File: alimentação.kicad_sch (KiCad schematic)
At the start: 10 parts, among them U2 LM317G, U3 AMS1117-5.0

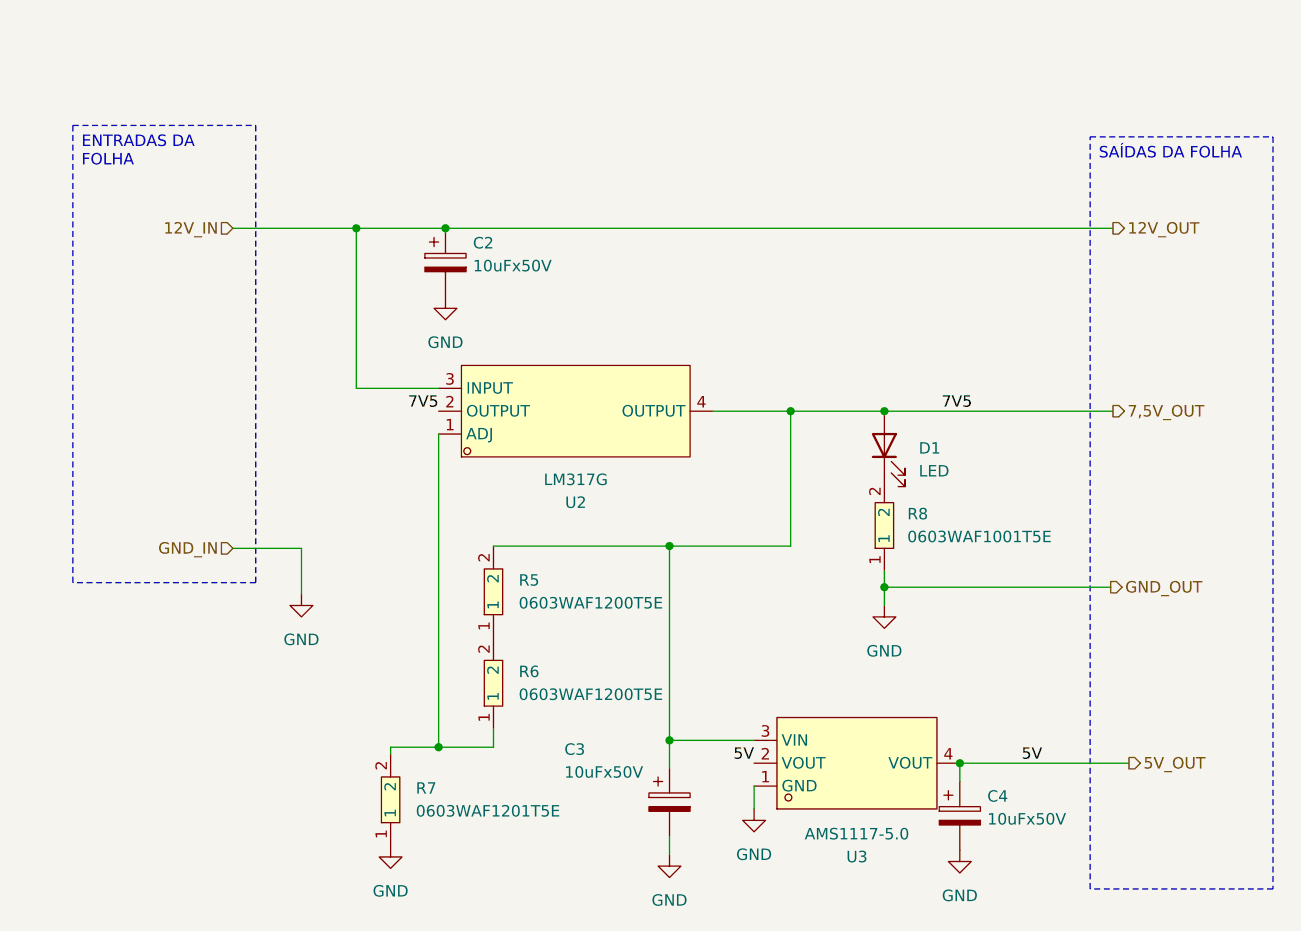
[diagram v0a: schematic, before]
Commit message: organização e legendas do esquemático
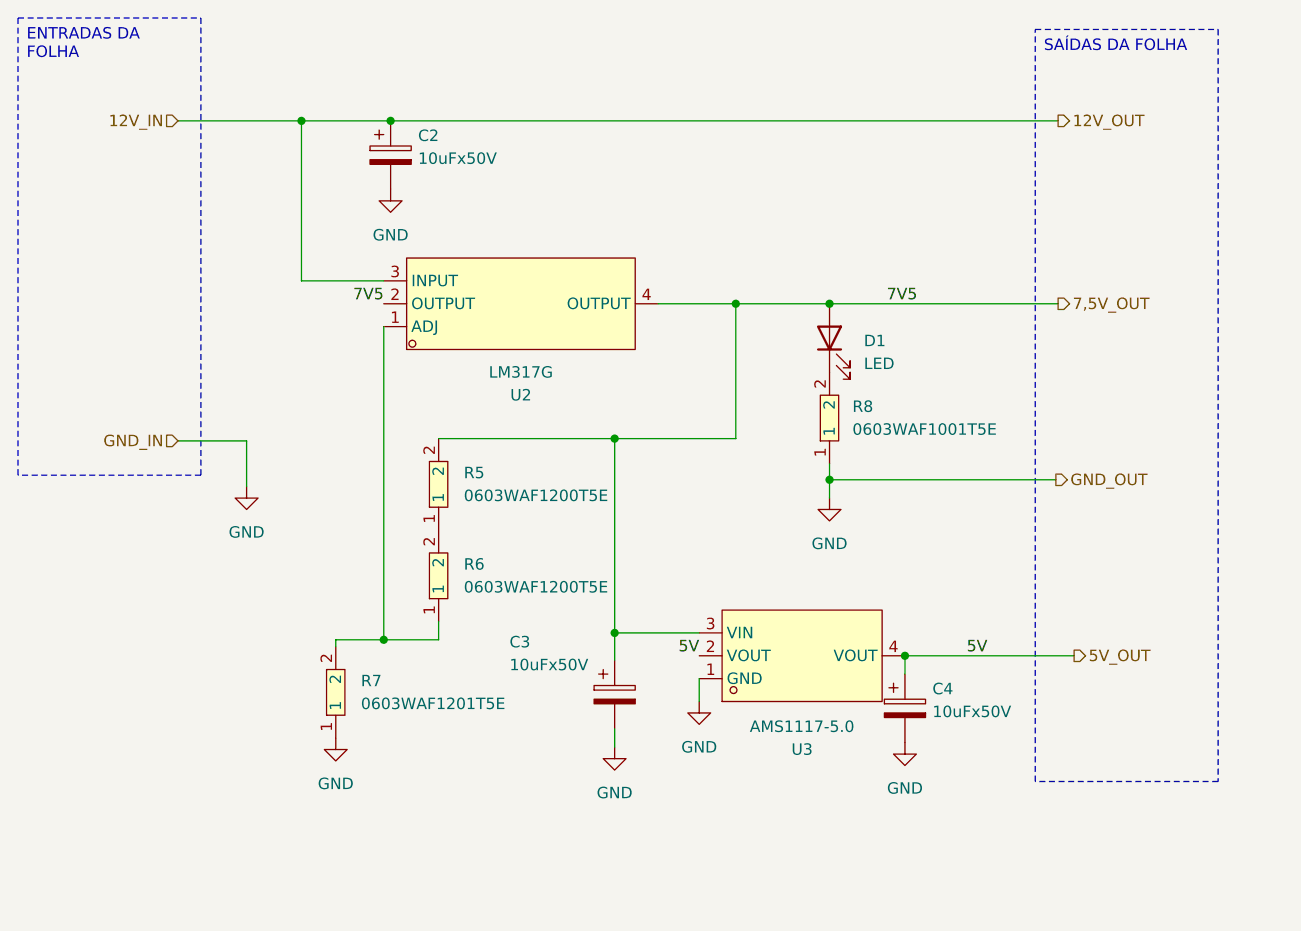
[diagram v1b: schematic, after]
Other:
- moved on the sheet: C2, C3, C4, D1, R5, R6, R7, R8, U2, U3
